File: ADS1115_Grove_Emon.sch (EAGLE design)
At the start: 20 parts, among them J1 ST-PJ-312, J2 ST-PJ-312, J3 GROVE-4P-2.0-SMD-FEMALE-REINF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, J4 GROVE-4P-2.0-SMD-FEMALE-REINF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, U1 ADS1115IDGST

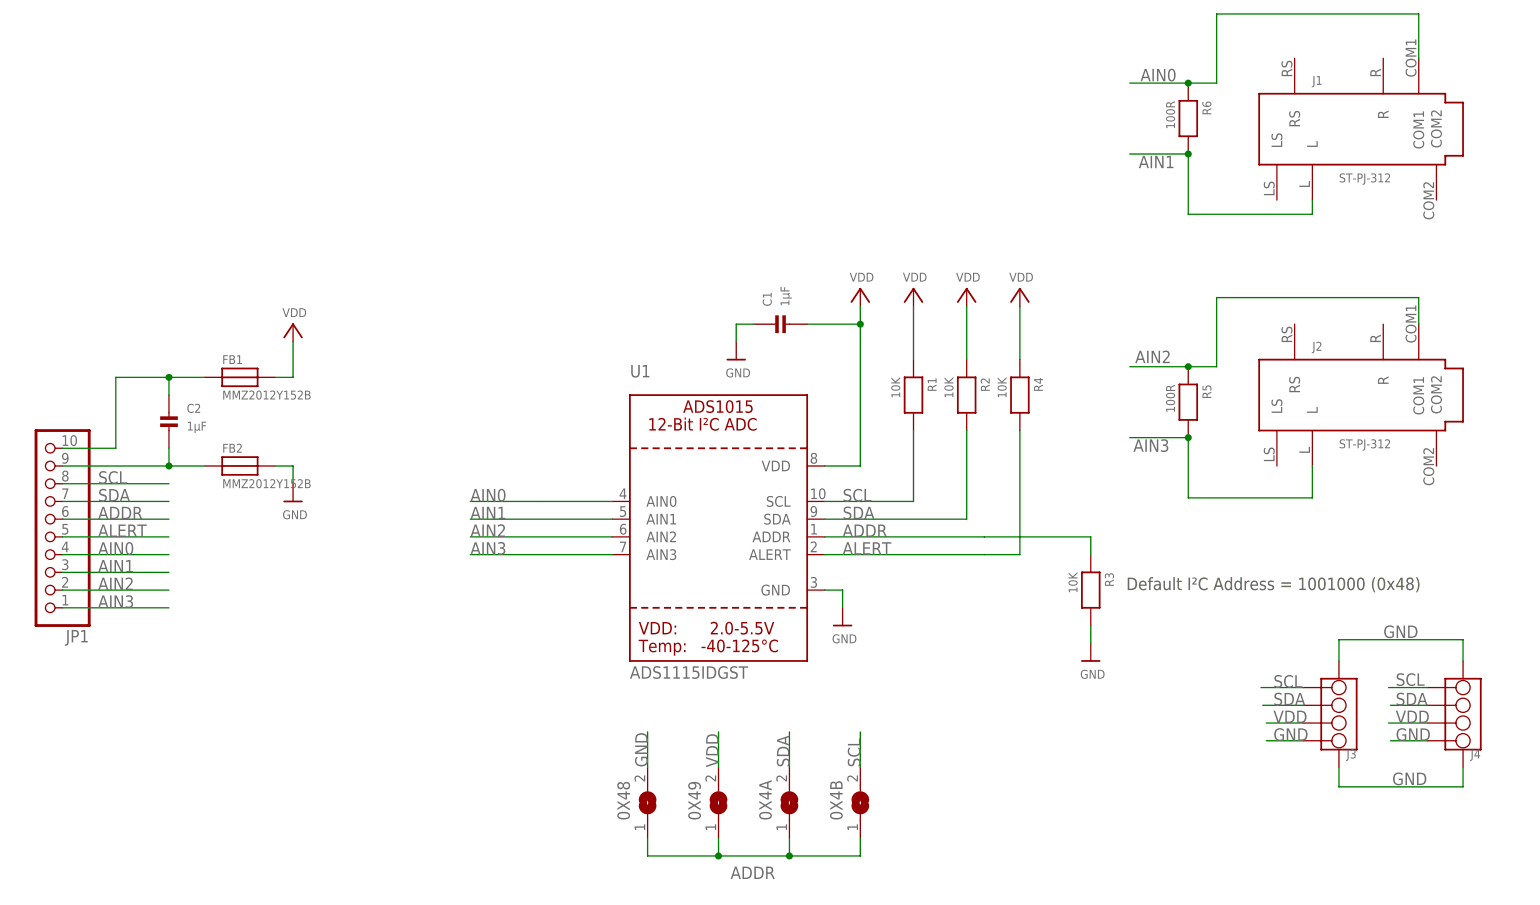
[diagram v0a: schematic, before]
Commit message: Fixed grove connector orientation
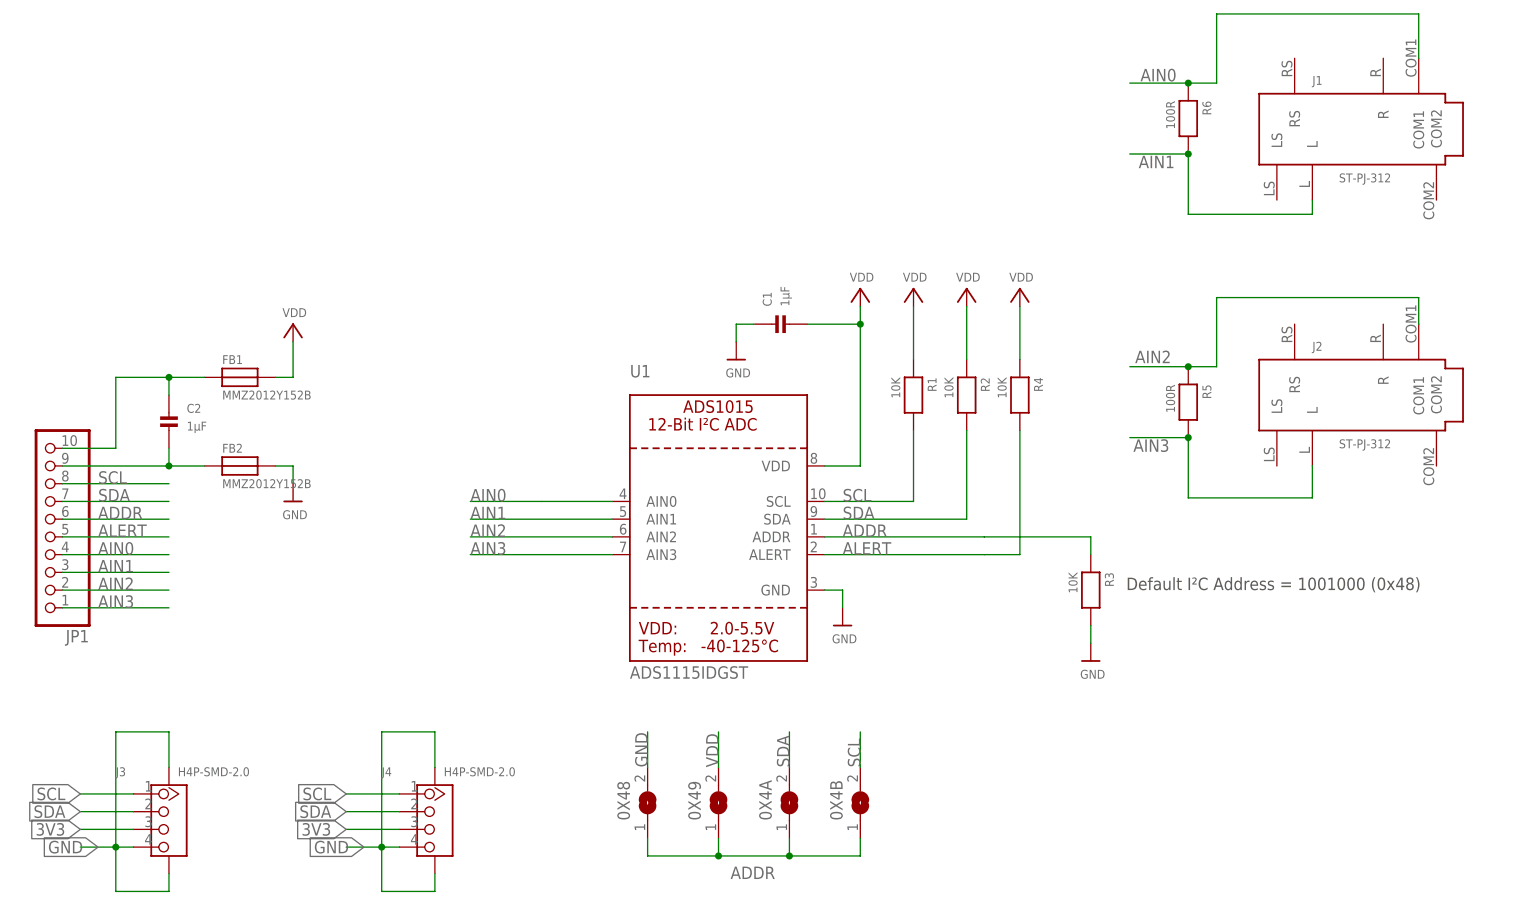
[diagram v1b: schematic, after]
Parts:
- J3, J4: value GROVE-4P-2.0-SMD-FEMALE-REINFORCE-3470090P1 -> H4P-SMD-2.0; device OPL:GROVE-4P-2.0-SMD-FEMALE-REINFORCE-3470090P1 -> Seeed-OPL-Connector:GROVE-CONNECTOR-SMD(4+2P-2.0)
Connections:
- new net 3V3: J3.3, J4.3
- net GND: now also J3.4, J4.4; no longer J3.1, J4.1
- net SCL: now also J3.1, J4.1; no longer J3.4, J4.4
- net SDA: now also J3.2, J4.2; no longer J3.3, J4.3
- net VDD: no longer J3.2, J4.2
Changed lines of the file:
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@@
 <clearance class="0" value="0.1524"/>
+</class>
+<class number="1" name="pwr" width="0.8128" drill="0">
+<clearance class="1" value="0.254"/>
 </class>
 </classes>
@@
 <part name="J1" library="Seeed-OPL-Connector" deviceset="AUDIO-JACK-6P-SMD(ST-PJ-312)" device="" value="ST-PJ-312"/>
 <part name="J2" library="Seeed-OPL-Connector" deviceset="AUDIO-JACK-6P-SMD(ST-PJ-312)" device="" value="ST-PJ-312"/>
-<part name="J3" library="OPL" deviceset="GROVE-4P-2.0-SMD-FEMALE-REINFORCE" device="-3470090P1"/>
-<part name="J4" library="OPL" deviceset="GROVE-4P-2.0-SMD-FEMALE-REINFORCE" device="-3470090P1"/>
 <part name="0X49" library="jumper" deviceset="SJ" device=""/>
 <part name="0X4A" library="jumper" deviceset="SJ" device=""/>
@@
 <part name="R5" library="microbuilder" deviceset="RESISTOR" device="0603" value="100R"/>
 <part name="R6" library="microbuilder" deviceset="RESISTOR" device="0603" value="100R"/>
+<part name="J3" library="Seeed-OPL-Connector" deviceset="GROVE-CONNECTOR-SMD(4+2P-2.0)" device="" value="H4P-SMD-2.0"/>
+<part name="J4" library="Seeed-OPL-Connector" deviceset="GROVE-CONNECTOR-SMD(4+2P-2.0)" device="" value="H4P-SMD-2.0"/>
 </parts>
 <sheets>
@@
 <instance part="J1" gate="G$1" x="215.9" y="154.94"/>
 <instance part="J2" gate="G$1" x="215.9" y="116.84"/>
-<instance part="J3" gate="J" x="213.36" y="71.12" smashed="yes" rot="R180">
-<attribute name="NAME" x="215.9" y="66.04" size="1.27" layer="95" ratio="10" rot="R180"/>
-</instance>
-<instance part="J4" gate="J" x="231.14" y="71.12" smashed="yes" rot="R180">
-<attribute name="NAME" x="233.68" y="66.04" size="1.27" layer="95" ratio="10" rot="R180"/>
-</instance>
 <instance part="0X49" gate="1" x="124.46" y="58.42" rot="R90"/>
 <instance part="0X4A" gate="1" x="134.62" y="58.42" rot="R90"/>
@@
 <instance part="R5" gate="G$1" x="191.77" y="115.824" rot="R270"/>
 <instance part="R6" gate="G$1" x="191.77" y="156.464" rot="R270"/>
+<instance part="J3" gate="G$1" x="45.72" y="55.88"/>
+<instance part="J4" gate="G$1" x="83.82" y="55.88"/>
 </instances>
 <busses>
@@
 </segment>
 <segment>
-<pinref part="J3" gate="J" pin="SS2"/>
-<wire x1="213.36" y1="78.74" x2="213.36" y2="81.788" width="0.1524" layer="91"/>
-<wire x1="213.36" y1="81.788" x2="231.14" y2="81.788" width="0.1524" layer="91"/>
-<pinref part="J4" gate="J" pin="SS2"/>
-<wire x1="231.14" y1="78.74" x2="231.14" y2="81.788" width="0.1524" layer="91"/>
-<label x="219.71" y="82.042" size="1.778" layer="95"/>
-</segment>
-<segment>
-<pinref part="J3" gate="J" pin="SS1"/>
-<wire x1="213.36" y1="63.5" x2="213.36" y2="60.706" width="0.1524" layer="91"/>
-<pinref part="J4" gate="J" pin="SS1"/>
-<wire x1="213.36" y1="60.706" x2="231.14" y2="60.706" width="0.1524" layer="91"/>
-<wire x1="231.14" y1="60.706" x2="231.14" y2="63.5" width="0.1524" layer="91"/>
-<label x="220.98" y="60.96" size="1.778" layer="95"/>
-</segment>
-<segment>
-<pinref part="J3" gate="J" pin="1"/>
-<wire x1="208.28" y1="67.31" x2="202.946" y2="67.31" width="0.1524" layer="91"/>
-<label x="203.962" y="67.31" size="1.778" layer="95"/>
-</segment>
-<segment>
-<label x="221.488" y="67.31" size="1.778" layer="95"/>
-<pinref part="J4" gate="J" pin="1"/>
-<wire x1="226.06" y1="67.31" x2="220.726" y2="67.31" width="0.1524" layer="91"/>
+<label x="35.56" y="52.07" size="1.778" layer="95" rot="R180" xref="yes"/>
+<pinref part="J3" gate="G$1" pin="4"/>
+<wire x1="40.64" y1="52.07" x2="38.1" y2="52.07" width="0.1524" layer="91"/>
+<pinref part="J3" gate="G$1" pin="SS1"/>
+<wire x1="38.1" y1="52.07" x2="33.02" y2="52.07" width="0.1524" layer="91"/>
+<wire x1="45.72" y1="63.5" x2="45.72" y2="68.58" width="0.1524" layer="91"/>
+<wire x1="45.72" y1="68.58" x2="38.1" y2="68.58" width="0.1524" layer="91"/>
+<wire x1="38.1" y1="68.58" x2="38.1" y2="52.07" width="0.1524" layer="91"/>
+<junction x="38.1" y="52.07"/>
+<pinref part="J3" gate="G$1" pin="SS2"/>
+<wire x1="45.72" y1="48.26" x2="45.72" y2="45.72" width="0.1524" layer="91"/>
+<wire x1="45.72" y1="45.72" x2="38.1" y2="45.72" width="0.1524" layer="91"/>
+<wire x1="38.1" y1="45.72" x2="38.1" y2="52.07" width="0.1524" layer="91"/>
+</segment>
+<segment>
+<label x="73.66" y="52.07" size="1.778" layer="95" rot="R180" xref="yes"/>
+<pinref part="J4" gate="G$1" pin="4"/>
+<wire x1="78.74" y1="52.07" x2="76.2" y2="52.07" width="0.1524" layer="91"/>
+<pinref part="J4" gate="G$1" pin="SS1"/>
+<wire x1="76.2" y1="52.07" x2="71.12" y2="52.07" width="0.1524" layer="91"/>
+<wire x1="83.82" y1="63.5" x2="83.82" y2="68.58" width="0.1524" layer="91"/>
+<wire x1="83.82" y1="68.58" x2="76.2" y2="68.58" width="0.1524" layer="91"/>
+<wire x1="76.2" y1="68.58" x2="76.2" y2="52.07" width="0.1524" layer="91"/>
+<junction x="76.2" y="52.07"/>
+<pinref part="J4" gate="G$1" pin="SS2"/>
+<wire x1="83.82" y1="48.26" x2="83.82" y2="45.72" width="0.1524" layer="91"/>
+<wire x1="83.82" y1="45.72" x2="76.2" y2="45.72" width="0.1524" layer="91"/>
+<wire x1="76.2" y1="45.72" x2="76.2" y2="52.07" width="0.1524" layer="91"/>
 </segment>
 </net>
@@
 </segment>
 <segment>
-<pinref part="J3" gate="J" pin="4"/>
-<wire x1="208.28" y1="74.93" x2="202.184" y2="74.93" width="0.1524" layer="91"/>
-<label x="203.962" y="74.93" size="1.778" layer="95"/>
-</segment>
-<segment>
-<pinref part="J4" gate="J" pin="4"/>
-<wire x1="226.06" y1="74.93" x2="220.472" y2="74.93" width="0.1524" layer="91"/>
-<label x="221.488" y="75.184" size="1.778" layer="95"/>
+<label x="33.02" y="59.69" size="1.778" layer="95" rot="R180" xref="yes"/>
+<pinref part="J3" gate="G$1" pin="1"/>
+<wire x1="40.64" y1="59.69" x2="33.02" y2="59.69" width="0.1524" layer="91"/>
+</segment>
+<segment>
+<label x="71.12" y="59.69" size="1.778" layer="95" rot="R180" xref="yes"/>
+<pinref part="J4" gate="G$1" pin="1"/>
+<wire x1="78.74" y1="59.69" x2="71.12" y2="59.69" width="0.1524" layer="91"/>
 </segment>
 </net>
@@
 </segment>
 <segment>
-<label x="203.962" y="72.39" size="1.778" layer="95"/>
-<pinref part="J3" gate="J" pin="3"/>
-<wire x1="208.28" y1="72.39" x2="202.438" y2="72.39" width="0.1524" layer="91"/>
-</segment>
-<segment>
-<label x="221.488" y="72.39" size="1.778" layer="95"/>
-<pinref part="J4" gate="J" pin="3"/>
-<wire x1="226.06" y1="72.39" x2="220.726" y2="72.39" width="0.1524" layer="91"/>
+<label x="33.02" y="57.15" size="1.778" layer="95" rot="R180" xref="yes"/>
+<pinref part="J3" gate="G$1" pin="2"/>
+<wire x1="40.64" y1="57.15" x2="33.02" y2="57.15" width="0.1524" layer="91"/>
+</segment>
+<segment>
+<label x="71.12" y="57.15" size="1.778" layer="95" rot="R180" xref="yes"/>
+<pinref part="J4" gate="G$1" pin="2"/>
+<wire x1="78.74" y1="57.15" x2="71.12" y2="57.15" width="0.1524" layer="91"/>
 </segment>
 </net>
@@
 <label x="124.46" y="63.5" size="1.778" layer="95" rot="R90"/>
 </segment>
-<segment>
-<label x="203.962" y="69.85" size="1.778" layer="95"/>
-<pinref part="J3" gate="J" pin="2"/>
-<wire x1="208.28" y1="69.85" x2="202.946" y2="69.85" width="0.1524" layer="91"/>
-</segment>
-<segment>
-<pinref part="J4" gate="J" pin="2"/>
-<wire x1="226.06" y1="69.85" x2="220.472" y2="69.85" width="0.1524" layer="91"/>
-<label x="221.488" y="69.85" size="1.778" layer="95"/>
-</segment>
 </net>
 <net name="ALERT" class="0">
@@
 </segment>
 </net>
+<net name="3V3" class="1">
+<segment>
+<label x="33.02" y="54.61" size="1.778" layer="95" rot="R180" xref="yes"/>
+<pinref part="J3" gate="G$1" pin="3"/>
+<wire x1="40.64" y1="54.61" x2="33.02" y2="54.61" width="0.1524" layer="91"/>
+</segment>
+<segment>
+<label x="71.12" y="54.61" size="1.778" layer="95" rot="R180" xref="yes"/>
+<pinref part="J4" gate="G$1" pin="3"/>
+<wire x1="78.74" y1="54.61" x2="71.12" y2="54.61" width="0.1524" layer="91"/>
+</segment>
+</net>
